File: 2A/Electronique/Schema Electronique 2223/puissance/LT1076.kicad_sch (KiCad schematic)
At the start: 10 parts

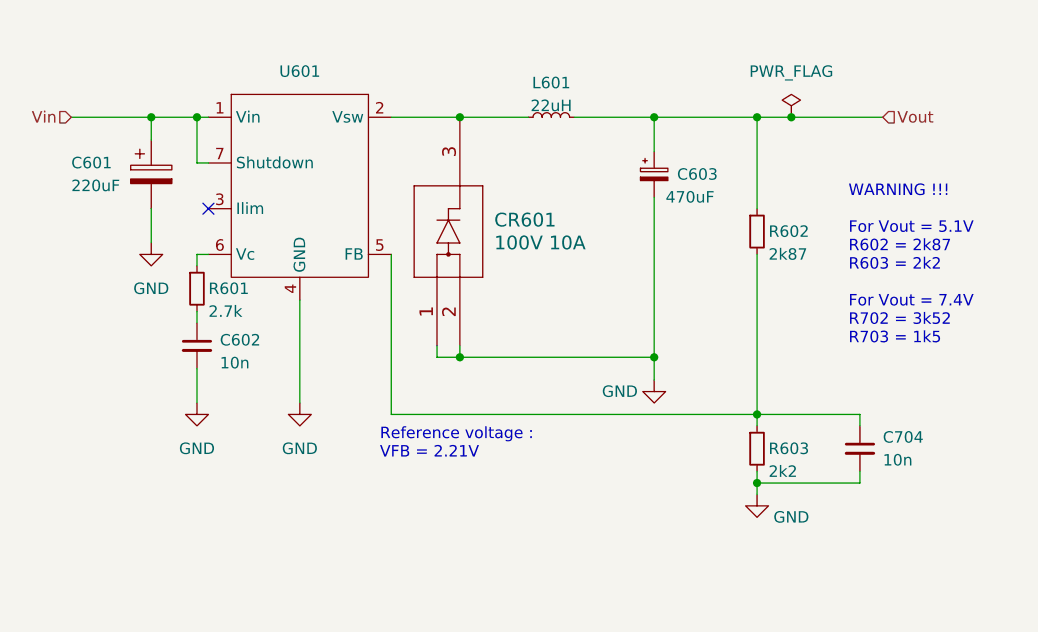
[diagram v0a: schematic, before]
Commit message: update puissance
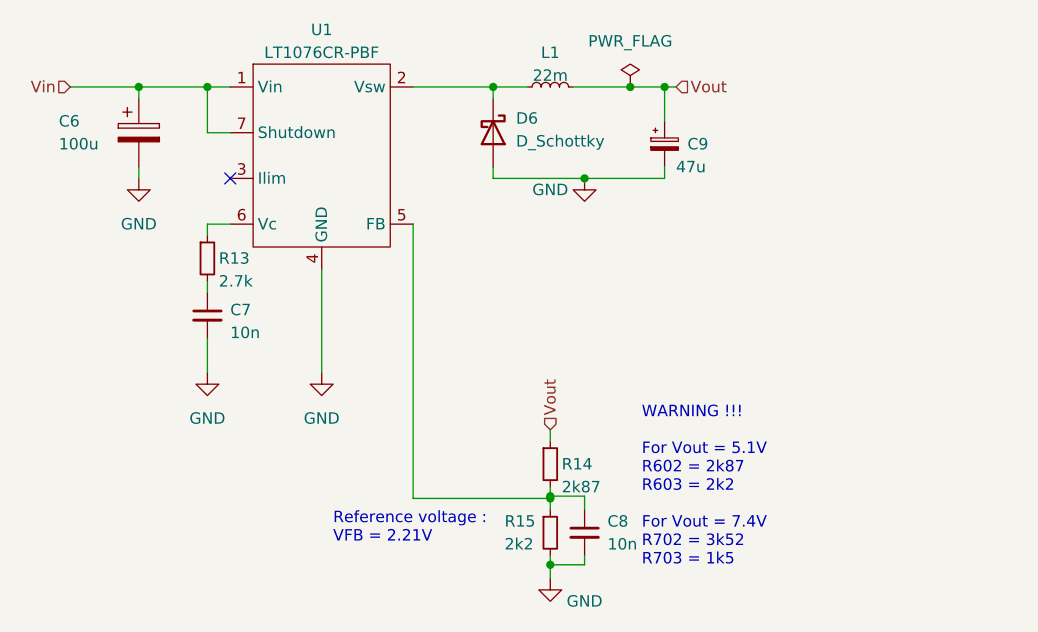
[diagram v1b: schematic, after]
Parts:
- removed C601: 220uF, Capacitor_SMD:C_0603_1608Metric_Pad1.08x0.95mm_HandSolder, symbol Device:C_Polarized
- removed C602: 10n, Capacitor_SMD:C_0603_1608Metric_Pad1.08x0.95mm_HandSolder, symbol Device:C_Small
- removed C603: 470uF, Capacitor_SMD:CP_Elec_10x10.5, symbol Device:C_Polarized_Small
- removed C704: 10n, symbol Device:C_Small
- removed CR601: 100V 10A, symbol custom:DST10100S
- removed L601: 22uH, Inductor_SMD:L_Wuerth_WE-PD-Typ-LS_Handsoldering, symbol Device:L_Small
- removed R601: 2.7k, Resistor_SMD:R_0603_1608Metric_Pad0.98x0.95mm_HandSolder, symbol Device:R_Small
- removed R602: 2k87, Resistor_SMD:R_0603_1608Metric_Pad0.98x0.95mm_HandSolder, symbol Device:R_Small
- removed R603: 2k2, Resistor_SMD:R_0603_1608Metric_Pad0.98x0.95mm_HandSolder, symbol Device:R_Small
- removed U601: ~, symbol custom:LT1076
- added C6: 100u, Capacitor_SMD:CP_Elec_6.3x7.7, symbol Device:C_Polarized
- added C7, C8: 10n, Capacitor_SMD:C_0402_1005Metric, symbol Device:C_Small
- added C9: 47u, Capacitor_SMD:CP_Elec_6.3x5.4, symbol Device:C_Polarized_Small
- added D6: D_Schottky, custom:DST10100S, symbol Device:D_Schottky
- added L1: 22m, Inductor_SMD:L_Changjiang_FNR8065S, symbol Device:L_Small
- added R13: 2.7k, Resistor_SMD:R_0402_1005Metric, symbol Device:R_Small
- added R14: 2k87, Resistor_SMD:R_0402_1005Metric, symbol Device:R_Small
- added R15: 2k2, Resistor_SMD:R_0402_1005Metric, symbol Device:R_Small
- added U1: LT1076CR-PBF, Package_TO_SOT_SMD:TO-263-7_TabPin4, symbol custom:LT1076
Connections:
- net GND: now also C6.2, C7.2, C8.2, C9.2, D6.2 (A), R15.2, U1.4 (GND)
- net Vin: now also C6.1, U1.1 (Vin), U1.7 (Shutdown)
- net Vout: now also C9.1, L1.2, R14.1
- new net: D6.1 (K), L1.1, U1.2 (Vsw)
- new net: C8.1, R14.2, R15.1, U1.5 (FB)
- new net: R13.1, U1.6 (Vc)
- new net: C7.1, R13.2
